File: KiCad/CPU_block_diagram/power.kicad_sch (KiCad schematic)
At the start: 0 parts

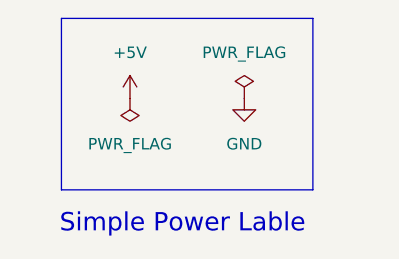
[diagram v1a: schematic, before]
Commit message: vault backup: 2025-12-30 00:26:07
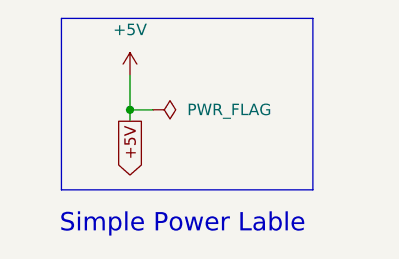
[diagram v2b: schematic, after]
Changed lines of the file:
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@@
+		)
+	)
+	(junction
+		(at 25.4 29.21)
+		(diameter 0)
+		(color 0 0 0 0)
+	)
+	(wire
+		(pts
+			(xy 25.4 29.21) (xy 25.4 25.4)
+		)
+		(stroke
+			(width 0)
+			(type default)
+		)
+	)
+	(wire
+		(pts
+			(xy 27.94 29.21) (xy 25.4 29.21)
+		)
+		(stroke
+			(width 0)
+			(type default)
+		)
+	)
+	(wire
+		(pts
+			(xy 25.4 29.21) (xy 25.4 30.48)
+		)
+		(stroke
+			(width 0)
+			(type default)
+		)
+	)
+	(global_label "+5V"
+		(shape output)
+		(at 25.4 30.48 270)
+		(fields_autoplaced yes)
+		(effects
+			(font
+				(size 1.27 1.27)
+			)
+			(justify right)
+		)
+		(property "Intersheetrefs" "${INTERSHEET_REFS}"
+			(at 25.4 37.3357 90)
+			(effects
+				(font
+					(size 1.27 1.27)
+				)
+				(justify right)
+				(hide yes)
+			)
 		)
 	)
 	(symbol
-		(lib_id "power:+5V")
-		(at 25.4 27.94 0)
+		(lib_id "power:PWR_FLAG")
+		(at 27.94 29.21 270)
 		(unit 1)
 		(exclude_from_sim no)
@@
 		(dnp no)
 		(fields_autoplaced yes)
-		(property "Reference" "#PWR07"
-			(at 25.4 31.75 0)
+		(property "Reference" "#FLG01"
+			(at 29.845 29.21 0)
+			(effects
+				(font
+					(size 1.27 1.27)
+				)
+				(hide yes)
+			)
+		)
+		(property "Value" "PWR_FLAG"
+			(at 31.75 29.2099 90)
+			(effects
+				(font
+					(size 1.27 1.27)
+				)
+				(justify left)
+			)
+		)
+		(property "Footprint" ""
+			(at 27.94 29.21 0)
+			(effects
+				(font
+					(size 1.27 1.27)
+				)
+				(hide yes)
+			)
+		)
+		(property "Datasheet" "~"
+			(at 27.94 29.21 0)
+			(effects
+				(font
+					(size 1.27 1.27)
+				)
+				(hide yes)
+			)
+		)
+		(property "Description" "Special symbol for telling ERC where power comes from"
+			(at 27.94 29.21 0)
+			(effects
+				(font
+					(size 1.27 1.27)
+				)
+				(hide yes)
+			)
+		)
+		(pin "1"
+		)
+		(instances
+			(project ""
+				(path "/5324683e-15fd-4fa9-8f28-7726564ef1dc/73188991-6c99-42c3-a6c7-3d96f653db2d"
+					(reference "#FLG01")
+					(unit 1)
+				)
+			)
+		)
+	)
+	(symbol
+		(lib_id "power:+5V")
+		(at 25.4 25.4 0)
+		(unit 1)
+		(exclude_from_sim no)
+		(in_bom yes)
+		(on_board yes)
+		(dnp no)
+		(fields_autoplaced yes)
+		(property "Reference" "#PWR02"
+			(at 25.4 29.21 0)
 			(effects
 				(font
@@
 		)
 		(property "Value" "+5V"
-			(at 25.4 22.86 0)
+			(at 25.4 20.32 0)
 			(effects
 				(font
@@
 		)
 		(property "Footprint" ""
-			(at 25.4 27.94 0)
+			(at 25.4 25.4 0)
 			(effects
 				(font
@@
 		)
 		(property "Datasheet" ""
-			(at 25.4 27.94 0)
+			(at 25.4 25.4 0)
 			(effects
 				(font
@@
 		)
 		(property "Description" "Power symbol creates a global label with name \"+5V\""
-			(at 25.4 27.94 0)
+			(at 25.4 25.4 0)
 			(effects
 				(font
@@
 			(project "CPU_block_diagram"
 				(path "/5324683e-15fd-4fa9-8f28-7726564ef1dc/73188991-6c99-42c3-a6c7-3d96f653db2d"
-					(reference "#PWR07")
+					(reference "#PWR02")
 					(unit 1)
 				)
-			)
-		)
-	)
-	(symbol
-		(lib_id "power:PWR_FLAG")
-		(at 25.4 27.94 180)
-		(unit 1)
-		(exclude_from_sim no)
-		(in_bom yes)
-		(on_board yes)
-		(dnp no)
-		(fields_autoplaced yes)
-		(property "Reference" "#FLG01"
-			(at 25.4 29.845 0)
-			(effects
-				(font
-					(size 1.27 1.27)
-				)
-				(hide yes)
-			)
-		)
-		(property "Value" "PWR_FLAG"
-			(at 25.4 33.02 0)
-			(effects
-				(font
-					(size 1.27 1.27)
-				)
-			)
-		)
-		(property "Footprint" ""
-			(at 25.4 27.94 0)
-			(effects
-				(font
-					(size 1.27 1.27)
-				)
-				(hide yes)
-			)
-		)
-		(property "Datasheet" "~"
-			(at 25.4 27.94 0)
-			(effects
-				(font
-					(size 1.27 1.27)
-				)
-				(hide yes)
-			)
-		)
-		(property "Description" "Special symbol for telling ERC where power comes from"
-			(at 25.4 27.94 0)
-			(effects
-				(font
-					(size 1.27 1.27)
-				)
-				(hide yes)
-			)
-		)
-		(pin "1"
-		)
-		(instances
-			(project "CPU_block_diagram"
-				(path "/5324683e-15fd-4fa9-8f28-7726564ef1dc/73188991-6c99-42c3-a6c7-3d96f653db2d"
-					(reference "#FLG01")
-					(unit 1)
-				)
-			)
-		)
-	)
-	(symbol
-		(lib_id "power:GND")
-		(at 38.1 27.94 0)
-		(unit 1)
-		(exclude_from_sim no)
-		(in_bom yes)
-		(on_board yes)
-		(dnp no)
-		(fields_autoplaced yes)
-		(property "Reference" "#PWR08"
-			(at 38.1 34.29 0)
-			(effects
-				(font
-					(size 1.27 1.27)
-				)
-				(hide yes)
-			)
-		)
-		(property "Value" "GND"
-			(at 38.1 33.02 0)
-			(effects
-				(font
-					(size 1.27 1.27)
-				)
-			)
-		)
-		(property "Footprint" ""
-			(at 38.1 27.94 0)
-			(effects
-				(font
-					(size 1.27 1.27)
-				)
-				(hide yes)
-			)
-		)
-		(property "Datasheet" ""
-			(at 38.1 27.94 0)
-			(effects
-				(font
-					(size 1.27 1.27)
-				)
-				(hide yes)
-			)
-		)
-		(property "Description" "Power symbol creates a global label with name \"GND\" , ground"
-			(at 38.1 27.94 0)
-			(effects
-				(font
-					(size 1.27 1.27)
-				)
-				(hide yes)
-			)
-		)
-		(pin "1"
-		)
-		(instances
-			(project "CPU_block_diagram"
-				(path "/5324683e-15fd-4fa9-8f28-7726564ef1dc/73188991-6c99-42c3-a6c7-3d96f653db2d"
-					(reference "#PWR08")
-					(unit 1)
-				)
-			)
-		)
-	)
-	(symbol
-		(lib_id "power:PWR_FLAG")
-		(at 38.1 27.94 0)
-		(unit 1)
-		(exclude_from_sim no)
-		(in_bom yes)
-		(on_board yes)
-		(dnp no)
-		(fields_autoplaced yes)
-		(property "Reference" "#FLG02"
-			(at 38.1 26.035 0)
-			(effects
-				(font
-					(size 1.27 1.27)
-				)
-				(hide yes)
-			)
-		)
-		(property "Value" "PWR_FLAG"
-			(at 38.1 22.86 0)
-			(effects
-				(font
-					(size 1.27 1.27)
-				)
-			)
-		)
-		(property "Footprint" ""
-			(at 38.1 27.94 0)
-			(effects
-				(font
-					(size 1.27 1.27)
-				)
-				(hide yes)
-			)
-		)
-		(property "Datasheet" "~"
-			(at 38.1 27.94 0)
-			(effects
-				(font
-					(size 1.27 1.27)
-				)
-				(hide yes)
-			)
-		)
-		(property "Description" "Special symbol for telling ERC where power comes from"
-			(at 38.1 27.94 0)
-			(effects
-				(font
-					(size 1.27 1.27)
-				)
-				(hide yes)
-			)
-		)
-		(pin "1"
-		)
-		(instances
-			(project "CPU_block_diagram"
-				(path "/5324683e-15fd-4fa9-8f28-7726564ef1dc/73188991-6c99-42c3-a6c7-3d96f653db2d"
-					(reference "#FLG02")
-					(unit 1)
-				)

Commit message: vault backup: 2025-12-30 22:01:07
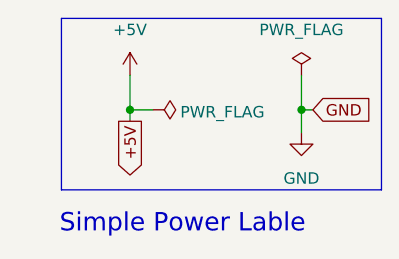
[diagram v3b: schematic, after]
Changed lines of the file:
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@@
 	(rectangle
 		(start 17.78 19.05)
-		(end 45.72 38.1)
+		(end 53.34 38.1)
 		(stroke
 			(width 0)
@@
 		(color 0 0 0 0)
 	)
+	(junction
+		(at 44.45 29.21)
+		(diameter 0)
+		(color 0 0 0 0)
+	)
+	(wire
+		(pts
+			(xy 44.45 25.4) (xy 44.45 29.21)
+		)
+		(stroke
+			(width 0)
+			(type default)
+		)
+	)
 	(wire
 		(pts
@@
 	(wire
 		(pts
+			(xy 45.72 29.21) (xy 44.45 29.21)
+		)
+		(stroke
+			(width 0)
+			(type default)
+		)
+	)
+	(wire
+		(pts
 			(xy 27.94 29.21) (xy 25.4 29.21)
 		)
@@
 			(width 0)
 			(type default)
+		)
+	)
+	(wire
+		(pts
+			(xy 44.45 29.21) (xy 44.45 31.75)
+		)
+		(stroke
+			(width 0)
+			(type default)
+		)
+	)
+	(global_label "GND"
+		(shape input)
+		(at 45.72 29.21 0)
+		(fields_autoplaced yes)
+		(effects
+			(font
+				(size 1.27 1.27)
+			)
+			(justify left)
+		)
+		(property "Intersheetrefs" "${INTERSHEET_REFS}"
+			(at 52.5757 29.21 0)
+			(effects
+				(font
+					(size 1.27 1.27)
+				)
+				(justify left)
+				(hide yes)
+			)
 		)
 	)
@@
 				(justify right)
 				(hide yes)
+			)
+		)
+	)
+	(symbol
+		(lib_id "power:GND")
+		(at 44.45 31.75 0)
+		(unit 1)
+		(exclude_from_sim no)
+		(in_bom yes)
+		(on_board yes)
+		(dnp no)
+		(fields_autoplaced yes)
+		(property "Reference" "#PWR05"
+			(at 44.45 38.1 0)
+			(effects
+				(font
+					(size 1.27 1.27)
+				)
+				(hide yes)
+			)
+		)
+		(property "Value" "GND"
+			(at 44.45 36.83 0)
+			(effects
+				(font
+					(size 1.27 1.27)
+				)
+			)
+		)
+		(property "Footprint" ""
+			(at 44.45 31.75 0)
+			(effects
+				(font
+					(size 1.27 1.27)
+				)
+				(hide yes)
+			)
+		)
+		(property "Datasheet" ""
+			(at 44.45 31.75 0)
+			(effects
+				(font
+					(size 1.27 1.27)
+				)
+				(hide yes)
+			)
+		)
+		(property "Description" "Power symbol creates a global label with name \"GND\" , ground"
+			(at 44.45 31.75 0)
+			(effects
+				(font
+					(size 1.27 1.27)
+				)
+				(hide yes)
+			)
+		)
+		(pin "1"
+		)
+		(instances
+			(project ""
+				(path "/5324683e-15fd-4fa9-8f28-7726564ef1dc/73188991-6c99-42c3-a6c7-3d96f653db2d"
+					(reference "#PWR05")
+					(unit 1)
+				)
 			)
 		)
@@
 		(on_board yes)
 		(dnp no)
-		(fields_autoplaced yes)
 		(property "Reference" "#FLG01"
 			(at 29.845 29.21 0)
@@
 		)
 		(property "Value" "PWR_FLAG"
-			(at 31.75 29.2099 90)
+			(at 30.988 29.464 90)
 			(effects
 				(font
@@
 		(dnp no)
 		(fields_autoplaced yes)
-		(property "Reference" "#PWR02"
+		(property "Reference" "#PWR04"
 			(at 25.4 29.21 0)
 			(effects
@@
 			(project "CPU_block_diagram"
 				(path "/5324683e-15fd-4fa9-8f28-7726564ef1dc/73188991-6c99-42c3-a6c7-3d96f653db2d"
-					(reference "#PWR02")
+					(reference "#PWR04")
 					(unit 1)
 				)
+			)
+		)
+	)
+	(symbol
+		(lib_id "power:PWR_FLAG")
+		(at 44.45 25.4 0)
+		(unit 1)
+		(exclude_from_sim no)
+		(in_bom yes)
+		(on_board yes)
+		(dnp no)
+		(fields_autoplaced yes)
+		(property "Reference" "#FLG02"
+			(at 44.45 23.495 0)
+			(effects
+				(font
+					(size 1.27 1.27)
+				)
+				(hide yes)
+			)
+		)
+		(property "Value" "PWR_FLAG"
+			(at 44.45 20.32 0)
+			(effects
+				(font
+					(size 1.27 1.27)
+				)
+			)
+		)
+		(property "Footprint" ""
+			(at 44.45 25.4 0)
+			(effects
+				(font
+					(size 1.27 1.27)
+				)
+				(hide yes)
+			)
+		)
+		(property "Datasheet" "~"
+			(at 44.45 25.4 0)
+			(effects
+				(font
+					(size 1.27 1.27)
+				)
+				(hide yes)
+			)
+		)
+		(property "Description" "Special symbol for telling ERC where power comes from"
+			(at 44.45 25.4 0)
+			(effects
+				(font
+					(size 1.27 1.27)
+				)
+				(hide yes)
+			)
+		)
+		(pin "1"
+		)
+		(instances
+			(project ""
+				(path "/5324683e-15fd-4fa9-8f28-7726564ef1dc/73188991-6c99-42c3-a6c7-3d96f653db2d"
+					(reference "#FLG02")
+					(unit 1)
+				)
